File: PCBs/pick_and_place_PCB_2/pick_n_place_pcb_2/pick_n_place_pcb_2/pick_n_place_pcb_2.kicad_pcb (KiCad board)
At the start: 2 copper layers, 63.2 x 43.1 mm, 8 parts, among them J1 Conn_01x04, J2 Conn_01x04, U1 Pick_and_place_pcb, U2 24AA02-OT

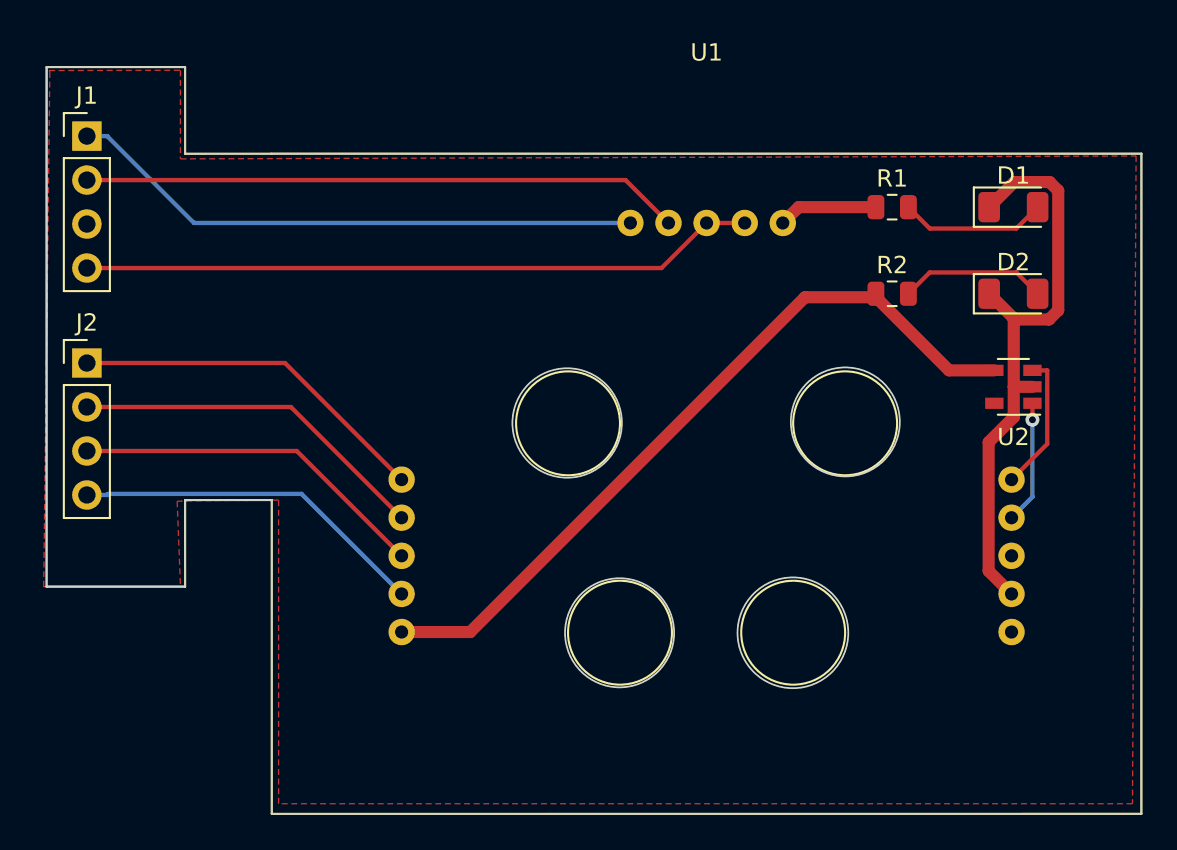
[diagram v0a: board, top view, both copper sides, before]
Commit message: modify kicad and freecad
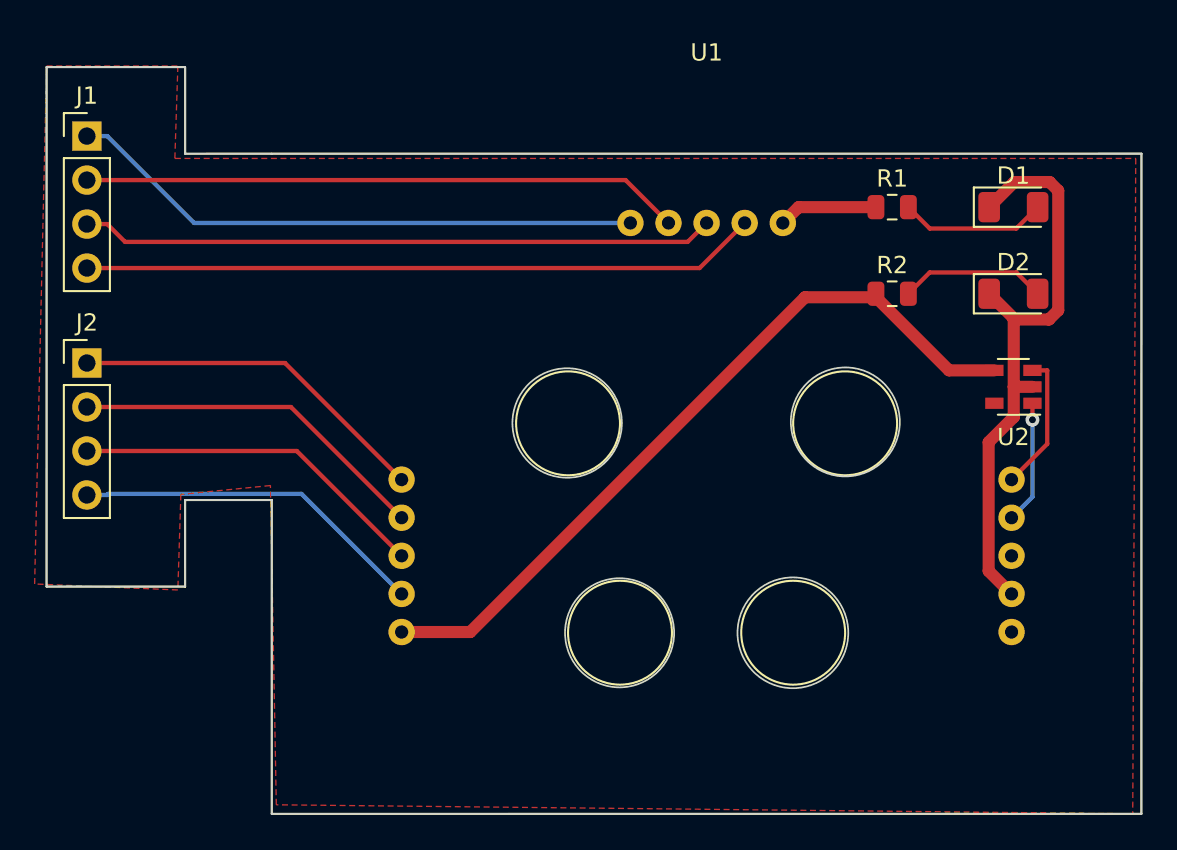
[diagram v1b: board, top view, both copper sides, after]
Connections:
- U1 pad 3: A2B -> A1B
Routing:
- net A1B: track 0.00 -> 36.7 mm
